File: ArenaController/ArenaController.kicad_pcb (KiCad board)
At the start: 2 copper layers, 80 x 90 mm, 30 parts, among them J1 RJ45, J2 RJ45, J4 RJ45, J5 RJ45, J6 RJ45, J8 Screw_Terminal_01x04, J9 Barrel_Jack_MountingPin, Q1 FS3400, Q2 FS3400, Q3 FS3400, Q4 FS3400, Q5 FS3400, Q6 Q_NMOS_GSD, U2 XT4140, U3 ESP32-Devkit_C_V4

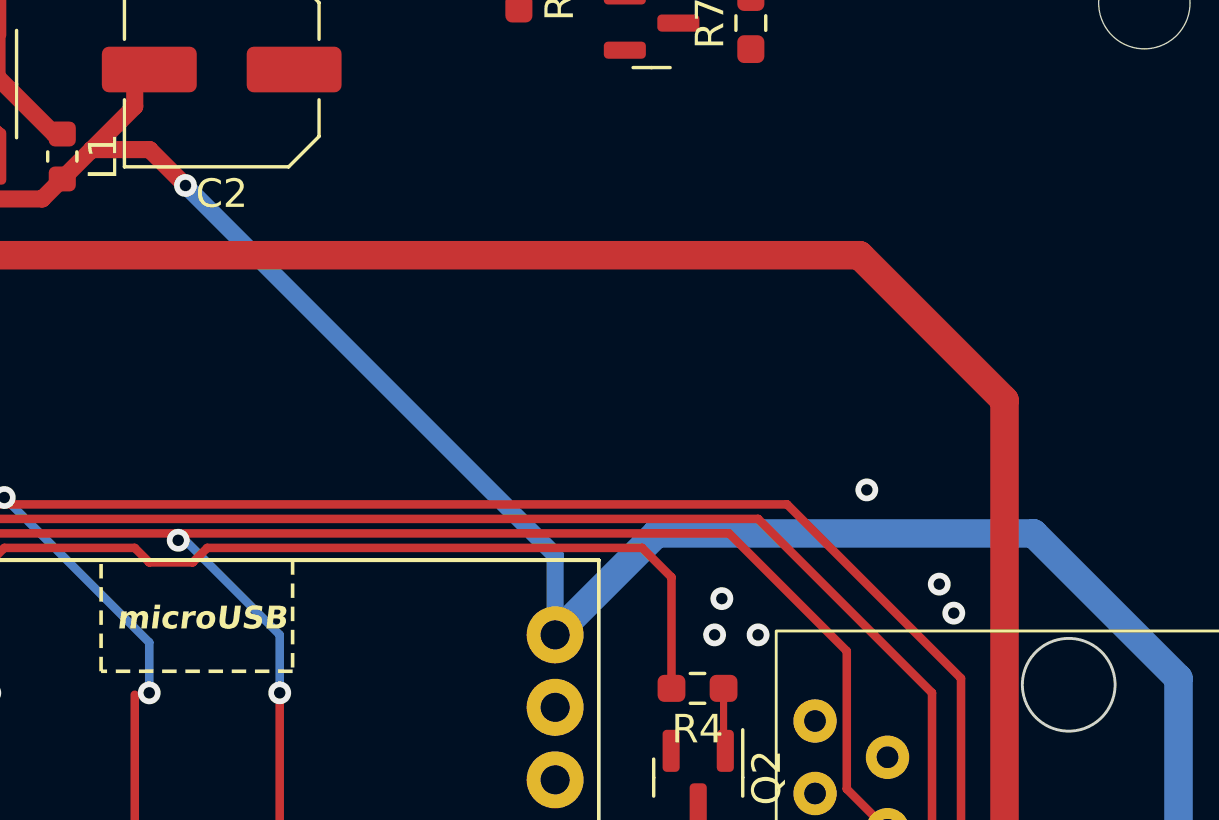
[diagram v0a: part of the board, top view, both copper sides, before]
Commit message: Release v.4 for April event.
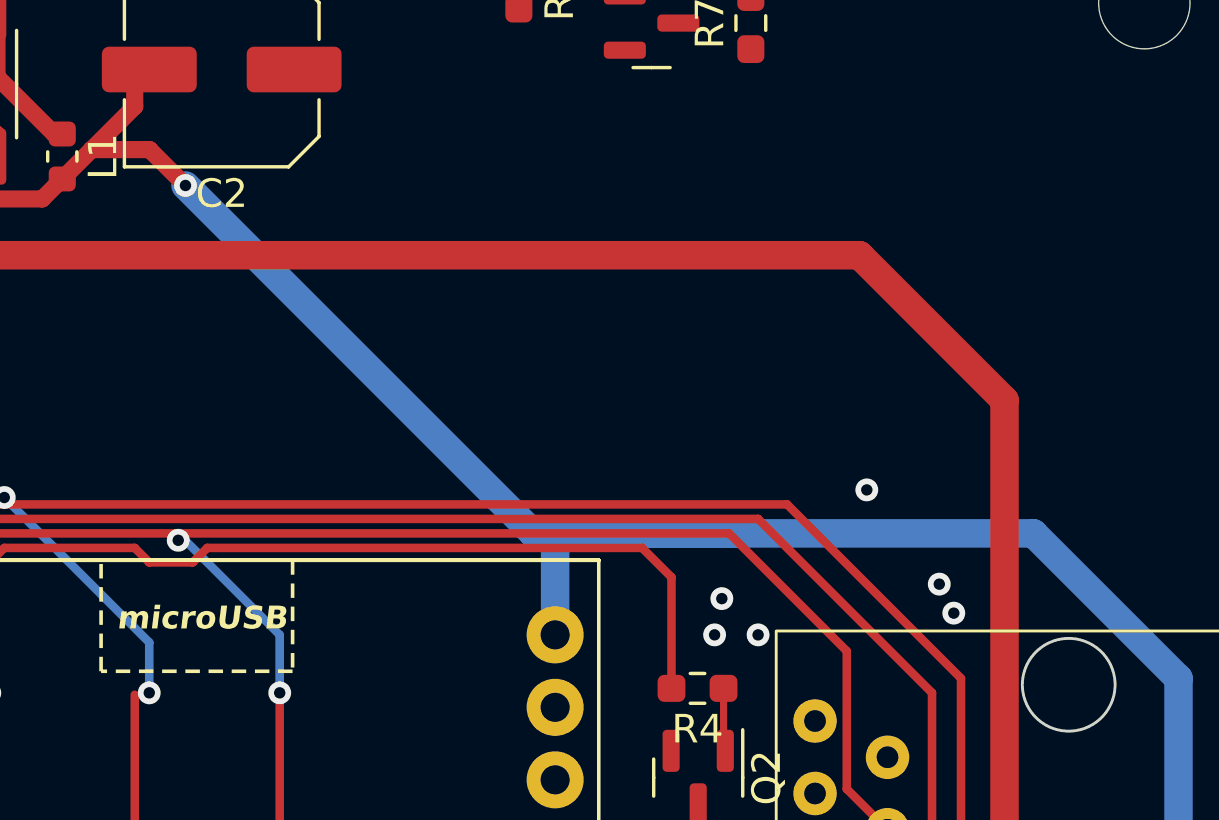
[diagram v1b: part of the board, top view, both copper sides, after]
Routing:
- net +5V: track 111.1 -> 117.5 mm
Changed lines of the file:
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@@
   (gr_text "TRANS RIGHTS\nTRANS FIGHTS" (at 125.476 128.778) (layer "B.Mask")
     (effects (font (face "Sushi Sans") (size 2 2) (thickness 0.5) bold) (justify left bottom mirror))
-    (render_cache "TRANS RIGHTS\nTRANS FIGHTS" -0
+    (render_cache "TRANS RIGHTS\nTRANS FIGHTS" 0
       (polygon
         (pts
@@
   (segment (start 125.984 56.026416) (end 126.817084 56.8595) (width 0.6) (layer "F.Cu") (net 33))
   (via (at 136.398 56.388) (size 0.8) (drill 0.4) (layers "F.Cu" "B.Cu") (net 33))
-  (segment (start 149.352 72.136) (end 152.908 68.58) (width 1) (layer "B.Cu") (net 33))
   (segment (start 166.116 68.58) (end 171.196 73.66) (width 1) (layer "B.Cu") (net 33))
-  (segment (start 136.398 56.388) (end 149.352 69.342) (width 0.6) (layer "B.Cu") (net 33))
-  (segment (start 149.352 69.342) (end 149.352 72.136) (width 0.6) (layer "B.Cu") (net 33))
+  (segment (start 152.908 68.58) (end 149.606 68.58) (width 1) (layer "B.Cu") (net 33))
+  (segment (start 149.606 68.58) (end 149.352 68.834) (width 1) (layer "B.Cu") (net 33))
+  (segment (start 155.956 68.58) (end 166.116 68.58) (width 1) (layer "B.Cu") (net 33))
+  (segment (start 148.59 68.58) (end 149.606 68.58) (width 0.6) (layer "B.Cu") (net 33))
+  (segment (start 149.352 68.834) (end 149.352 72.136) (width 1) (layer "B.Cu") (net 33))
+  (segment (start 155.956 68.58) (end 148.59 68.58) (width 1) (layer "B.Cu") (net 33))
   (segment (start 171.196 121.412) (end 170.688 121.92) (width 1) (layer "B.Cu") (net 33))
-  (segment (start 152.908 68.58) (end 166.116 68.58) (width 1) (layer "B.Cu") (net 33))
+  (segment (start 152.908 68.58) (end 155.956 68.58) (width 1) (layer "B.Cu") (net 33))
   (segment (start 171.196 73.66) (end 171.196 121.412) (width 1) (layer "B.Cu") (net 33))
+  (segment (start 148.59 68.58) (end 136.398 56.388) (width 1) (layer "B.Cu") (net 33))
   (segment (start 114.8865 73.0785) (end 111.54 76.425) (width 0.3) (layer "F.Cu") (net 35))
   (segment (start 114.8865 72.136) (end 114.8865 73.0785) (width 0.3) (layer "F.Cu") (net 35))
